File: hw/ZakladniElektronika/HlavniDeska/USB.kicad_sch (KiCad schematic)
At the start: 18 parts, among them J2 USB_C_Receptacle_USB2.0, U13 TPD4E02B04DQA, U4 AP33772

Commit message: AHS-V1
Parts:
- J2: JLCPCB_CORRECTION 0;-1;0 -> 0;-3.5;0
- U13: JLCPCB_CORRECTION (none) -> 0;0;-90
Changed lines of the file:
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@@
       (effects (font (size 1.27 1.27)) hide)
     )
-    (property "JLCPCB_CORRECTION" "0;-1;0" (at 71.12 58.42 0)
+    (property "JLCPCB_CORRECTION" "0;-3.5;0" (at 71.12 58.42 0)
       (effects (font (size 1.27 1.27)) hide)
     )
@@
       (effects (font (size 1.27 1.27)) hide)
     )
+    (property "JLCPCB_CORRECTION" "0;0;-90" (at 96.52 92.71 0)
+      (effects (font (size 1.27 1.27)) hide)
+    )

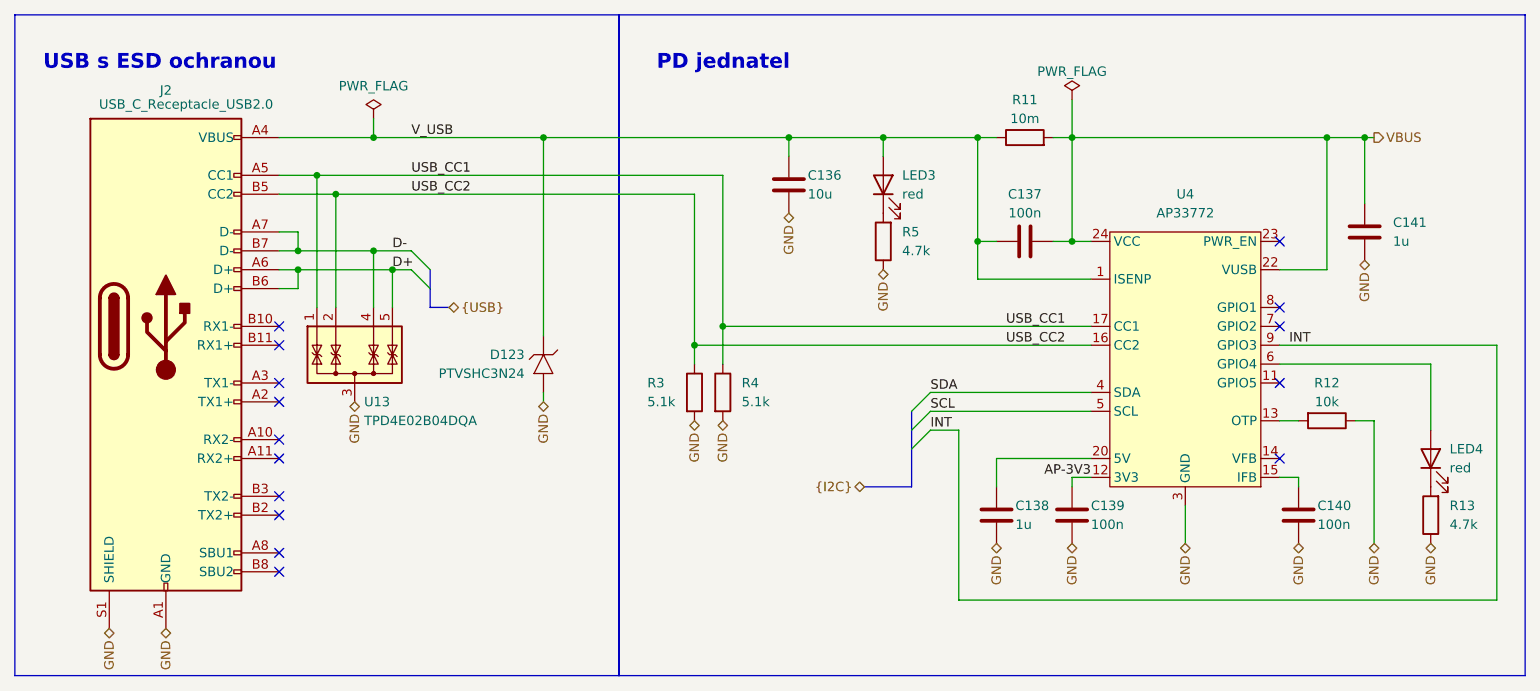
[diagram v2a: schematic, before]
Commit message: Hw PCB
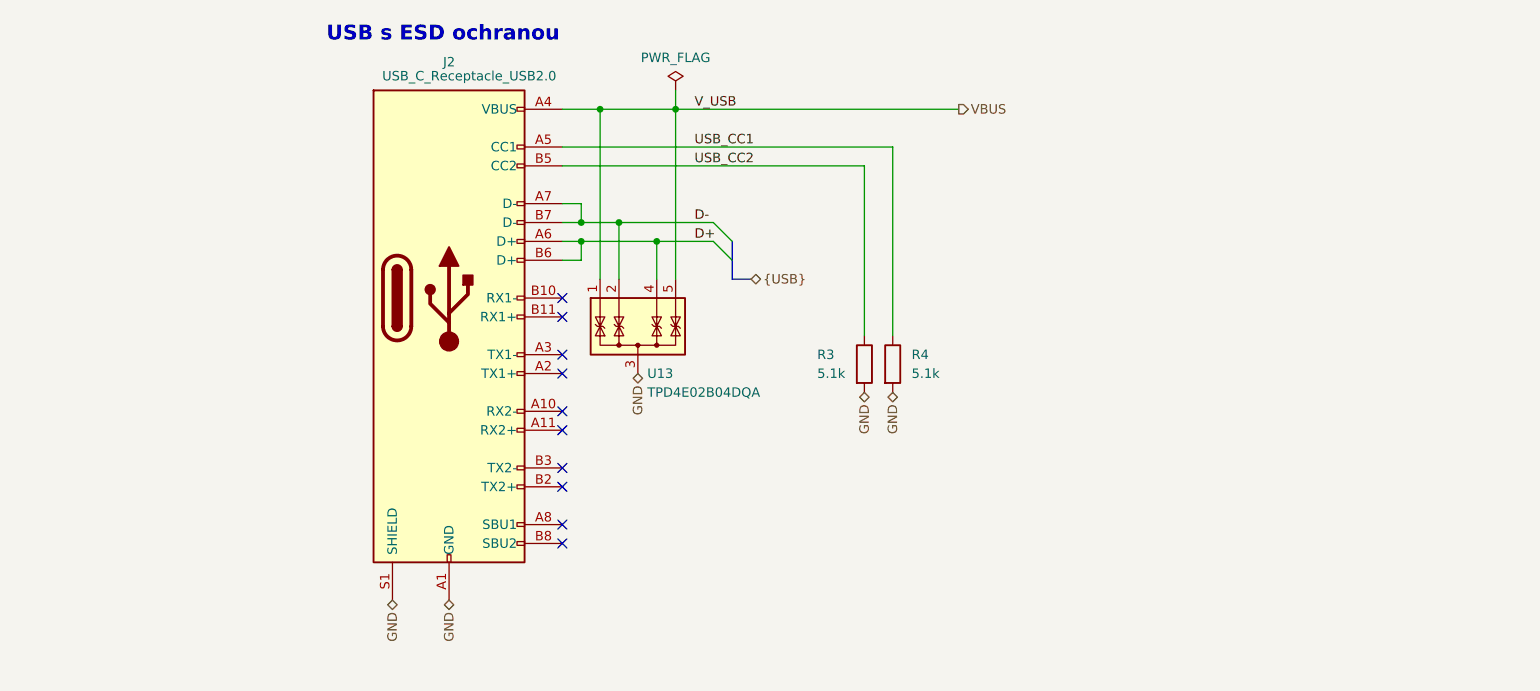
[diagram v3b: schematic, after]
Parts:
- removed C136: 10u, Capacitor_SMD:C_0805_2012Metric, symbol Device:C
- removed C137, C139, C140: 100n, Capacitor_SMD:C_0402_1005Metric, symbol Device:C
- removed C138, C141: 1u, Capacitor_SMD:C_0402_1005Metric, symbol Device:C
- removed D123: PTVSHC3N24, RKL-StandardPackages:DFN3-2x2, symbol RKL-Uncategorized:PTVSHC3N24
- removed LED3, LED4: red, LED_SMD:LED_0603_1608Metric, symbol Device:LED
- removed R11: 10m, Resistor_SMD:R_1206_3216Metric, symbol Device:R
- removed R12: 10k, Resistor_SMD:R_0402_1005Metric, symbol Device:R
- removed R13, R5: 4.7k, Resistor_SMD:R_0402_1005Metric, symbol Device:R
- removed U4: AP33772, Package_DFN_QFN:QFN-24-1EP_4x4mm_P0.5mm_EP2.6x2.6mm, symbol RKL-BusCnverters:AP33772
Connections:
- net V_USB is gone; now on net VBUS: J2.A4 (VBUS), J2.A9 (VBUS), J2.B4 (VBUS), J2.B9 (VBUS)
- net D+: now also U13.4 (IO3); no longer U13.5 (IO4)
- net D-: now also U13.2 (IO2); no longer U13.4 (IO3)
- net USB_CC1: no longer U13.1 (IO1)
- net USB_CC2: no longer U13.2 (IO2)
- net VBUS: now also U13.1 (IO1), U13.5 (IO4)
- no-connect marks 15 -> 10
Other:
- note removed: "PD jednatel"
- moved on the sheet: J2, R3, R4, U13
